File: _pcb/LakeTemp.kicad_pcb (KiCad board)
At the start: 2 copper layers, 98 x 70 mm, 50 parts, among them J1 Conn_01x06_Male, J2 Conn_01x03_Male, J3 Conn_01x02_Female, J4 Conn_01x14_Female, J5 Conn_01x04_Male, J6 Conn_01x06_Male, J7 Conn_01x02_Female, J8 Conn_01x03_Female, J9 Conn_01x02_Female, Q1 S8050, SW1 RESET, SW2 FLASH, U1 PCF8574, U2 ICL7660, U3 NCP1117-3.3_SOT223, U4 ESP-12E, U5 DS18B20

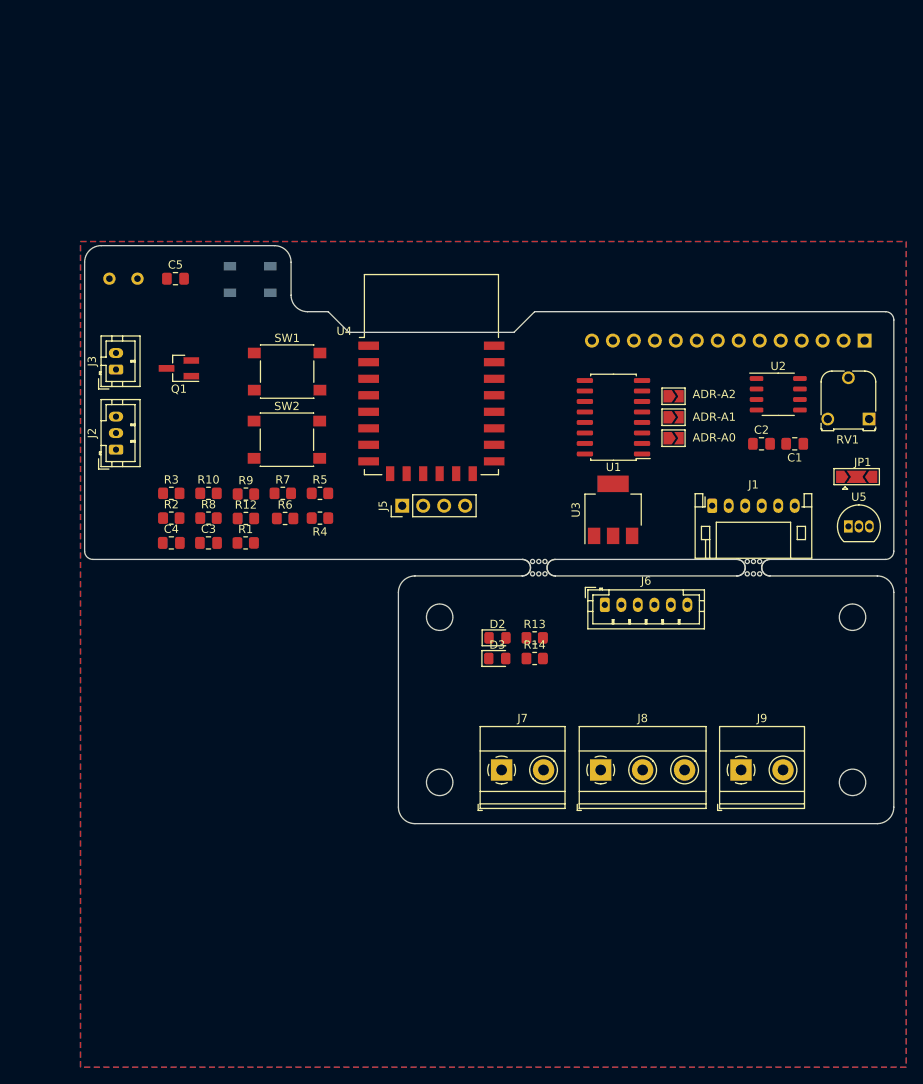
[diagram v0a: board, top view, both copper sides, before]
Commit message: Update PCB
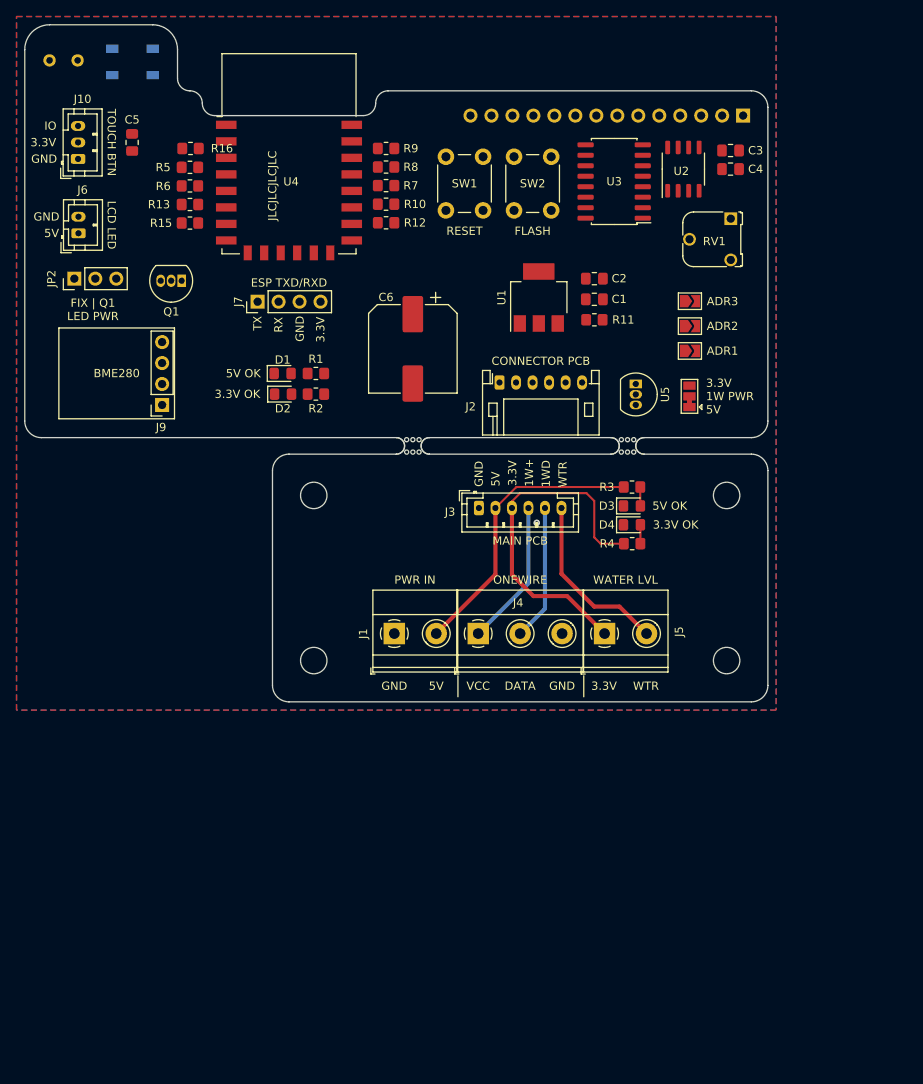
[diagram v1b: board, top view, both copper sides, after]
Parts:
- removed ADR-A0: SolderJumper_2_Open, Jumper:SolderJumper-2_P1.3mm_Open_TrianglePad1.0x1.5mm
- added ADR-A3: SolderJumper_2_Open, Jumper:SolderJumper-2_P1.3mm_Open_TrianglePad1.0x1.5mm, F.Cu at (188.1, 84.2)
- added C6: 1000uF, Capacitor_SMD:CP_Elec_10x10.5, F.Cu at (154.5, 90.0)
- added D4: PWR 3.3V, LED_SMD:LED_0805_2012Metric_Pad1.15x1.40mm_HandSolder, F.Cu at (181.0, 111.3)
- added D5: WS2812B, LED_SMD:LED_WS2812B_PLCC4_5.0x5.0mm_P3.2mm, B.Cu at (120.6, 55.2)
- added J10: Conn_01x03_Male, Connector_JST:JST_PH_B3B-PH-K_1x03_P2.00mm_Vertical, F.Cu at (114.0, 67.0)
- added JP2: SolderJumper_3_Open, Connector_PinHeader_2.54mm:PinHeader_1x03_P2.54mm_Vertical, F.Cu at (113.5, 81.5)
- added R15: 4,7k, Resistor_SMD:R_0805_2012Metric_Pad1.20x1.40mm_HandSolder, F.Cu at (127.5, 74.8)
- added R16: 10k, Resistor_SMD:R_0805_2012Metric_Pad1.20x1.40mm_HandSolder, F.Cu at (127.6, 65.7)
- C1, C2, C3, C4: value 10uF 50V -> 10uF
- D1: value WS2812B -> PWR 5V; footprint LED_SMD:LED_WS2812B_PLCC4_5.0x5.0mm_P3.2mm -> LED_SMD:LED_0805_2012Metric_Pad1.15x1.40mm_HandSolder; moved to F.Cu
- D2: value LED -> PWR 3.3V
- D3: value LED -> PWR 5V
- J1: value Conn_01x06_Male -> Conn_01x02_Female; footprint Connector_JST:JST_PH_S6B-PH-K_1x06_P2.00mm_Horizontal -> TerminalBlock_Phoenix:TerminalBlock_Phoenix_MKDS-1,5-2-5.08_1x02_P5.08mm_Horizontal
- J2: value Conn_01x03_Male -> Conn_01x06_Male; footprint Connector_JST:JST_PH_B3B-PH-K_1x03_P2.00mm_Vertical -> Connector_JST:JST_PH_S6B-PH-K_1x06_P2.00mm_Horizontal
- J3: value Conn_01x02_Female -> Conn_01x06_Male; footprint Connector_JST:JST_PH_B2B-PH-K_1x02_P2.00mm_Vertical -> Connector_JST:JST_PH_B6B-PH-K_1x06_P2.00mm_Vertical
- J4: value Conn_01x14_Female -> Conn_01x03_Female; footprint Connector_PinHeader_2.54mm:PinHeader_1x14_P2.54mm_Vertical -> TerminalBlock_Phoenix:TerminalBlock_Phoenix_MKDS-1,5-3-5.08_1x03_P5.08mm_Horizontal; moved to F.Cu
- J5: value Conn_01x04_Male -> Conn_01x02_Female; footprint Connector_PinHeader_2.54mm:PinHeader_1x04_P2.54mm_Vertical -> TerminalBlock_Phoenix:TerminalBlock_Phoenix_MKDS-1,5-2-5.08_1x02_P5.08mm_Horizontal
- J6: value Conn_01x06_Male -> Conn_01x02_Female; footprint Connector_JST:JST_PH_B6B-PH-K_1x06_P2.00mm_Vertical -> Connector_JST:JST_PH_B2B-PH-K_1x02_P2.00mm_Vertical
- J7: value Conn_01x02_Female -> Conn_01x04_Male; footprint TerminalBlock_Phoenix:TerminalBlock_Phoenix_MKDS-1,5-2-5.08_1x02_P5.08mm_Horizontal -> Connector_PinHeader_2.54mm:PinHeader_1x04_P2.54mm_Vertical
- J8: value Conn_01x03_Female -> Conn_01x14_Female; footprint TerminalBlock_Phoenix:TerminalBlock_Phoenix_MKDS-1,5-3-5.08_1x03_P5.08mm_Horizontal -> Connector_PinHeader_2.54mm:PinHeader_1x14_P2.54mm_Vertical; moved to B.Cu
- J9: value Conn_01x02_Female -> Conn_01x04_Female; footprint TerminalBlock_Phoenix:TerminalBlock_Phoenix_MKDS-1,5-2-5.08_1x02_P5.08mm_Horizontal -> Connector_PinSocket_2.54mm:PinSocket_1x04_P2.54mm_Vertical
- JP1: footprint Jumper:SolderJumper-3_P2.0mm_Open_TrianglePad1.0x1.5mm -> Jumper:SolderJumper-3_P1.3mm_Bridged12_Pad1.0x1.5mm
- Q1: footprint Package_TO_SOT_SMD:SOT-23_Handsoldering -> Package_TO_SOT_THT:TO-92_Inline
- R1, R3: value 4,7k -> 150
- R11: value R_PHOTO -> 4,7k; footprint OptoDevice:R_LDR_5.1x4.3mm_P3.4mm_Vertical -> Resistor_SMD:R_0805_2012Metric_Pad1.20x1.40mm_HandSolder; moved to F.Cu
- R12: value R -> 10k
- R13: value R -> 4,7k
- R14: value R -> GL5528; footprint Resistor_SMD:R_0805_2012Metric_Pad1.20x1.40mm_HandSolder -> OptoDevice:R_LDR_5.1x4.3mm_P3.4mm_Vertical; moved to B.Cu
- R2, R4: value 4,7k -> 68
- R8: value 10k -> 4,7k
- SW1, SW2: footprint Button_Switch_SMD:SW_Push_1P1T_NO_6x6mm_H9.5mm -> Button_Switch_THT:SW_PUSH_6mm_H5mm
- U1: value PCF8574 -> NCP1117-3.3_SOT223; footprint Package_SO:SO-16_5.3x10.2mm_P1.27mm -> Package_TO_SOT_SMD:SOT-223-3_TabPin2
- U3: value NCP1117-3.3_SOT223 -> PCF8574; footprint Package_TO_SOT_SMD:SOT-223-3_TabPin2 -> Package_SO:SO-16_5.3x10.2mm_P1.27mm
- moved R14 93.3 mm to (110.5, 55.1)
- moved J9 82.9 mm to (124.1, 96.8), turned to 180 degrees
- moved C4 81.5 mm to (193.0, 68.2), turned to 180 degrees
- moved J8 81.1 mm to (194.5, 61.8), turned to 90 degrees
- moved C3 79.1 mm to (193.0, 66.0)
- moved J6 78.0 mm to (114.0, 76.0), turned to 90 degrees
- moved R13 67.1 mm to (127.5, 72.5), turned to 180 degrees
- moved J7 63.9 mm to (135.7, 84.3), turned to 90 degrees
- moved R11 58.9 mm to (176.5, 86.5)
- moved J4 58.7 mm to (162.4, 124.5), turned to 0 degrees
- moved R3 55.8 mm to (181.1, 106.7)
- moved R8 47.6 mm to (151.3, 68.0), turned to 180 degrees
- moved J2 47.2 mm to (165.0, 94.1), turned to 0 degrees
- moved J3 47.0 mm to (162.5, 109.3), turned to 0 degrees
- moved SW2 46.9 mm to (171.3, 66.7), turned to 270 degrees
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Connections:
- ADR-A1 pad 1: PCF_A1 -> PCF_A0
- ADR-A2 pad 1: PCF_A2 -> PCF_A1
- C1 pad 1: GND -> +5V
- C1 pad 2: Net-(C1-Pad2) -> GND
- C2 pad 1: Net-(C2-Pad1) -> +3V3
- C2 pad 2: Net-(C2-Pad2) -> GND
- C3 pad 1: +5V -> Net-(C3-Pad1)
- C3 pad 2: GND -> Net-(C3-Pad2)
- C4 pad 1: +3V3 -> Net-(C4-Pad1)
- D1 pad 1: +5V -> GND
- D1 pad 2: (no net) -> Net-(D1-Pad2)
- J1 pad 2: +5V -> Net-(J1-Pad2)
- J2 pad 2: +3V3 -> +5V
- J2 pad 3: TOUCH_IO -> +3V3
- J3 pad 1: +5V -> GND
- J3 pad 2: Net-(J3-Pad2) -> Net-(J1-Pad2)
- J4 pad 1: GND -> Net-(J3-Pad4)
- J4 pad 2: +5V -> Net-(J3-Pad5)
- J4 pad 3: LCD_CONTRAST -> GND
- J5 pad 1: ESP_TX -> Net-(J3-Pad3)
- J5 pad 2: ESP_RX -> Net-(J3-Pad6)
- J6 pad 1: Net-(J6-Pad1) -> +5V
- J7 pad 1: Net-(J6-Pad1) -> ESP_TX
- J7 pad 2: Net-(J6-Pad2) -> ESP_RX
- J8 pad 1: Net-(J6-Pad4) -> GND
- J8 pad 2: Net-(J6-Pad5) -> +5V
- J8 pad 3: GND -> LCD_CONTRAST
- J9 pad 1: Net-(J6-Pad3) -> +3V3
- J9 pad 2: Net-(J6-Pad6) -> GND
- Q1 pad 3: Net-(J3-Pad2) -> Net-(JP2-Pad3)
- R1 pad 1: +3V3 -> +5V
- R1 pad 2: SDA -> Net-(D1-Pad2)
- R11 pad 1: +3V3 -> ONEWIRE_PWR
- R11 pad 2: LDR -> ONEWIRE_BUS
- R12 pad 1: LDR -> GND
- R12 pad 2: GND -> Net-(R12-Pad2)
- R13 pad 1: Net-(J6-Pad2) -> WATER_LEVEL
- R13 pad 2: Net-(D2-Pad2) -> GND
- R14 pad 1: Net-(J6-Pad3) -> +3V3
- R14 pad 2: Net-(D3-Pad2) -> LDR
- R2 pad 2: SCL -> Net-(D2-Pad2)
- R3 pad 1: +5V -> Net-(J1-Pad2)
- R3 pad 2: LCD_LED -> Net-(D3-Pad2)
- R4 pad 1: +3V3 -> Net-(J3-Pad3)
- R4 pad 2: ONEWIRE_BUS -> Net-(D4-Pad2)
- R8 pad 1: GND -> +3V3
- R8 pad 2: Net-(R8-Pad2) -> SDA
- R9 pad 1: WATER_LEVEL -> +3V3
- R9 pad 2: GND -> SCL
- RV1 pad 1: Net-(C1-Pad2) -> Net-(C4-Pad1)
- U1 pad 1: PCF_A0 -> GND
- U1 pad 2: PCF_A1 -> +3V3
- U1 pad 3: PCF_A2 -> +5V
- U2 pad 1: (no net) -> Net-(U2-Pad1)
- U2 pad 2: Net-(C2-Pad1) -> Net-(C3-Pad1)
- U2 pad 4: Net-(C2-Pad2) -> Net-(C3-Pad2)
- U2 pad 5: Net-(C1-Pad2) -> Net-(C4-Pad1)
- U2 pad 6: (no net) -> Net-(U2-Pad6)
- U2 pad 7: (no net) -> Net-(U2-Pad7)
- U3 pad 1: GND -> PCF_A0
- U3 pad 2: +3V3 -> PCF_A1
- U3 pad 3: +5V -> PCF_A2
- U4 pad 10: (no net) -> Net-(U4-Pad10)
- U4 pad 11: (no net) -> Net-(U4-Pad11)
- U4 pad 12: (no net) -> Net-(U4-Pad12)
- U4 pad 13: (no net) -> Net-(U4-Pad13)
- U4 pad 14: (no net) -> Net-(U4-Pad14)
- U4 pad 16: Net-(R8-Pad2) -> Net-(R12-Pad2)
- U4 pad 9: (no net) -> Net-(U4-Pad9)
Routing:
- net Net-(J3-Pad3): track 0.00 -> 42.8 mm
- net Net-(J1-Pad2): track 0.00 -> 34.8 mm
- net Net-(J3-Pad6): track 0.00 -> 22.3 mm
- net Net-(J3-Pad4): track 0.00 -> 17.7 mm
- net Net-(J3-Pad5): track 0.00 -> 16.5 mm
- net Net-(D3-Pad2): track 0.00 -> 2.29 mm
- net Net-(D4-Pad2): track 0.00 -> 2.29 mm
- net GND: vias 0 -> 1
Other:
- board size 98 x 70 mm -> 90 x 82 mm
- board text added: "1W+"
- board text added: "1WD"
- board text added: "3.3V"
- board text added: "3.3V 1W PWR 5V"
- board text added: "3.3V OK"
- board text added: "5V"
- board text added: "5V OK"
- board text added: "ADR1"
- board text added: "ADR2"
- board text added: "ADR3"
- board text added: "BME280"
- board text added: "CONNECTOR PCB"
- board text added: "DATA"
- board text added: "ESP TXD/RXD"
- board text added: "FIX | Q1 LED PWR"
- board text added: "FLASH"
- board text added: "GND"
- board text added: "IO"
- board text added: "JLCJLCJLCJLC"
- board text added: "LCD LED"
- board text added: "MAIN PCB"
- board text added: "ONEWIRE"
- board text added: "PWR IN"
- board text added: "RESET"
- board text added: "RX"
- board text added: "STATUS"
- board text added: "TOUCH BTN"
- board text added: "TX"
- board text added: "VCC"
- board text added: "WATER LVL"
- board text added: "WTR"
